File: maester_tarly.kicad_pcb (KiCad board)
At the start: 4 copper layers, 72 x 62.4 mm, 126 parts, among them J101 Micro_SD_Card_Det, J102 USB_B_Micro, J103 USB_A, J104 Conn_01x06, J105 Conn_01x10, J106 RJ45_Amphenol_RJMG1BD3B8K1ANR, J107 DF40GB(1.5)-48DS-0.4V, J108 DF40GB(1.5)-48DS-0.4V, J109 DF40GB(1.5)-48DS-0.4V, J110 DF40GB(1.5)-48DS-0.4V, U1 SAM9X60, U2 W971GG6SB-18, U3 MCP16501, U501 KSZ8081RNA, Y401 32.768kHz, Y402 DSC1001, Y501 DSC1001

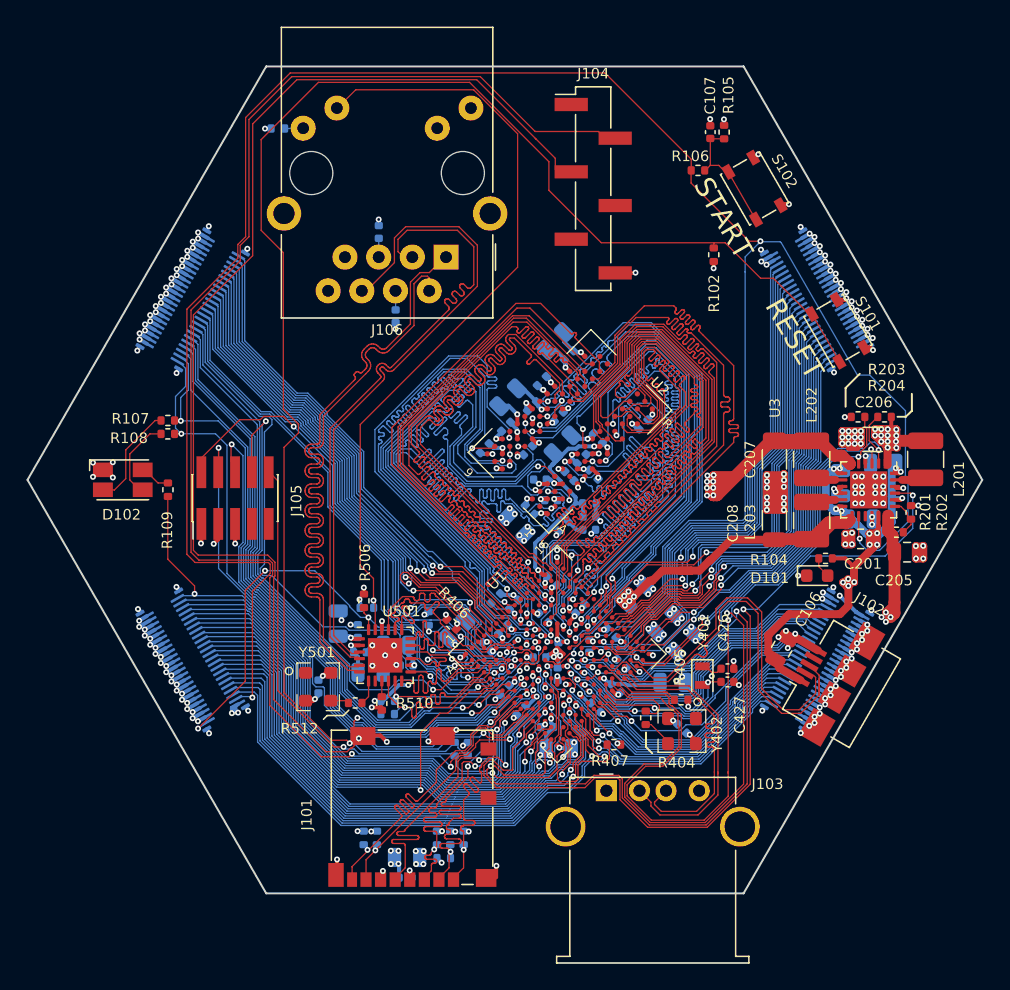
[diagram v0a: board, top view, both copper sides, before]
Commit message: Clean DRC
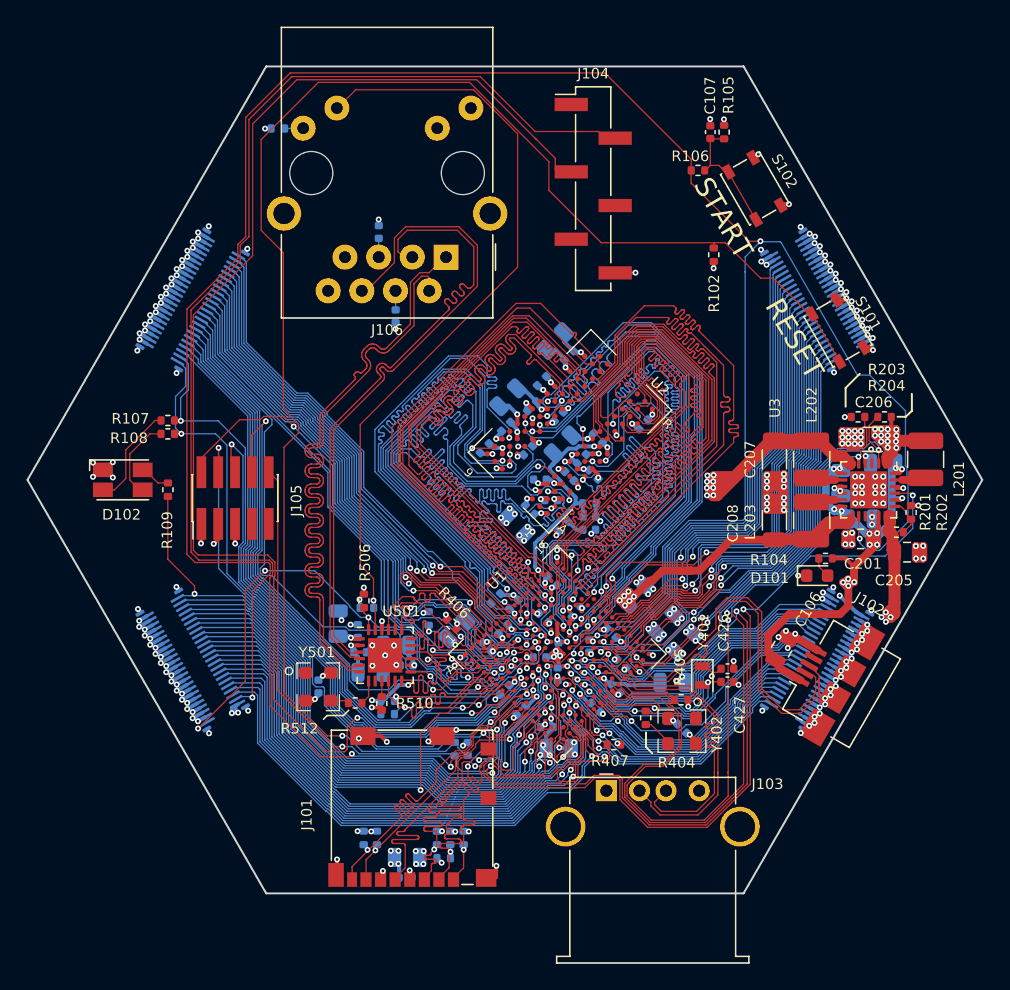
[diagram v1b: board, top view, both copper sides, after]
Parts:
- moved C416 0.39 mm to (123.4, 141.2)
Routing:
- net +5V: track 139.4 -> 121.9 mm
- net /CPU_IO/PHY_TXD0: track 12.0 -> 8.97 mm
- net +3V3: track 56.8 -> 57.8 mm
- net /a21: track 42.9 -> 42.3 mm
- net GND: track 216.6 -> 216.0 mm
